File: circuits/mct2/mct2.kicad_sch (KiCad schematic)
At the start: 36 parts

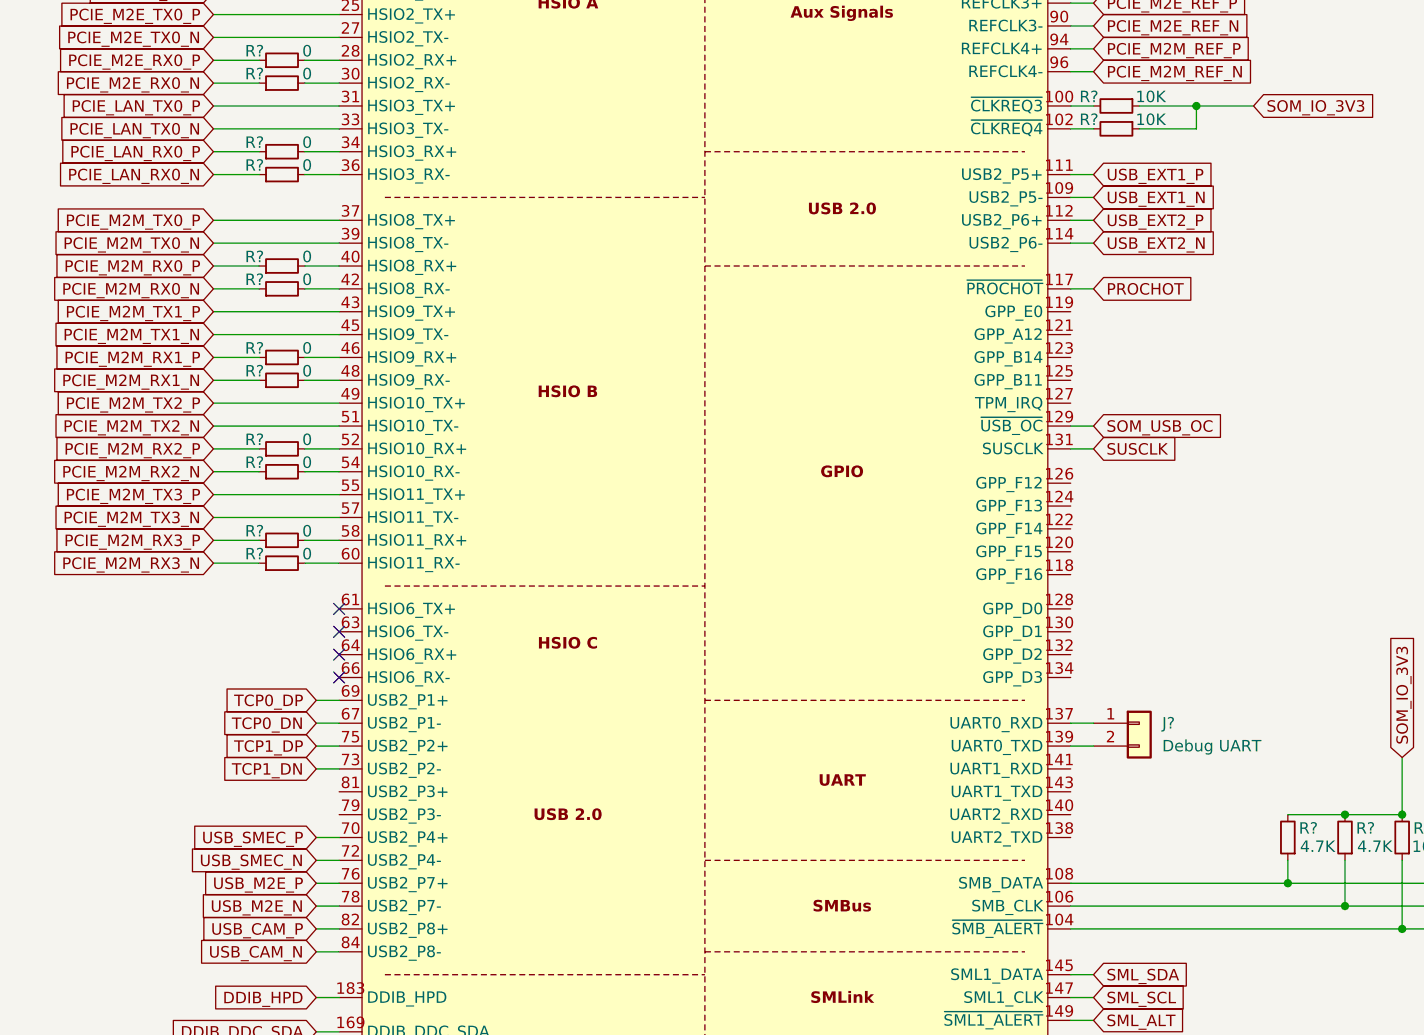
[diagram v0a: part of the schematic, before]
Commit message: Sep 5, 2024 2
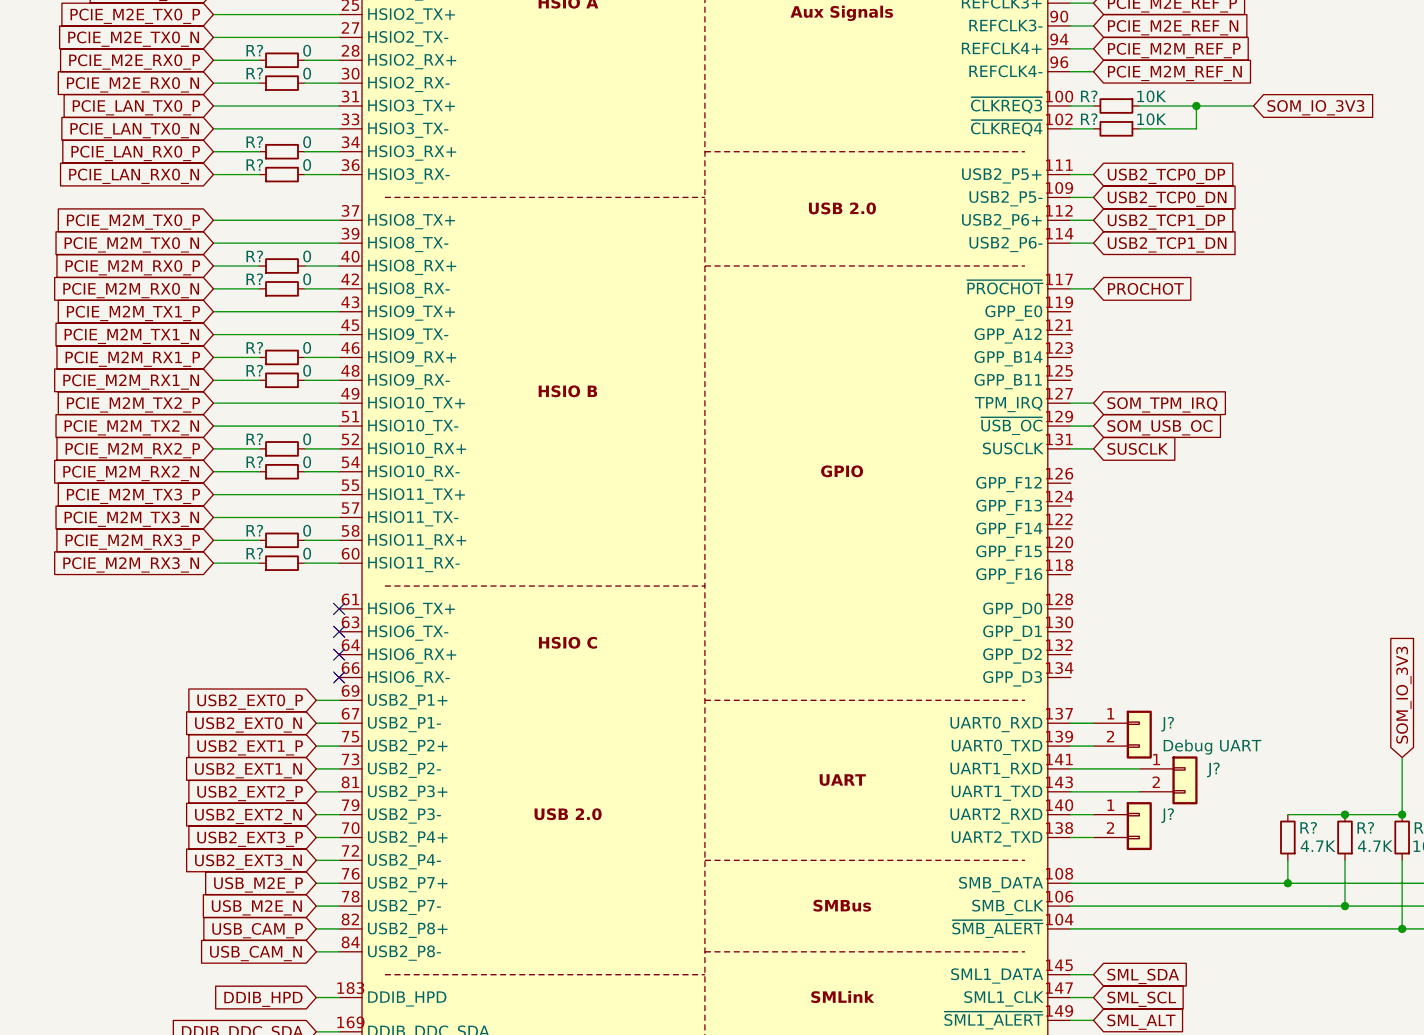
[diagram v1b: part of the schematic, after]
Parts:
- added J? (x2): ~, Connector_PinHeader_2.54mm:PinHeader_1x02_P2.54mm_Vertical, symbol Connector_Generic:Conn_01x02
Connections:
- net SOM_TPM_IRQ: now reaches A1.127 (TPM_IRQ)
- net at A1.138 (UART2_TXD): now also J?.2 (Pin_2)
- net at A1.140 (UART2_RXD): now also J?.1 (Pin_1)
- net at A1.141 (UART1_RXD): now also J?.1 (Pin_1)
- net at A1.143 (UART1_TXD): now also J?.2 (Pin_2)
- net USB2_EXT2_N: now reaches A1.79 (USB2_P3-)
- net USB2_EXT2_P: now reaches A1.81 (USB2_P3+)
- net TCP0_DN renamed USB2_EXT0_N
- net TCP0_DP renamed USB2_EXT0_P
- net TCP1_DN renamed USB2_EXT1_N
- net TCP1_DP renamed USB2_EXT1_P
- net USB_EXT1_N renamed USB2_TCP0_DN
- net USB_EXT1_P renamed USB2_TCP0_DP
- net USB_EXT2_N renamed USB2_TCP1_DN
- net USB_EXT2_P renamed USB2_TCP1_DP
- net USB_SMEC_N renamed USB2_EXT3_N
- net USB_SMEC_P renamed USB2_EXT3_P
